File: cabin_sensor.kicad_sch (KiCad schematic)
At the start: 6 parts, among them J5 Внутр. коннектор вентилятора 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, Q2 AO3400

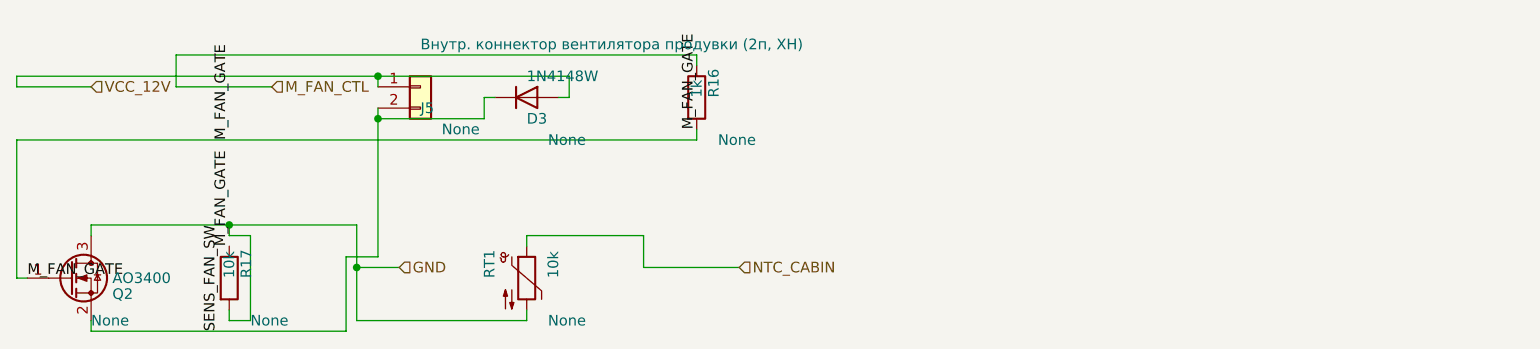
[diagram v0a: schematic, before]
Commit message: all unit test pass
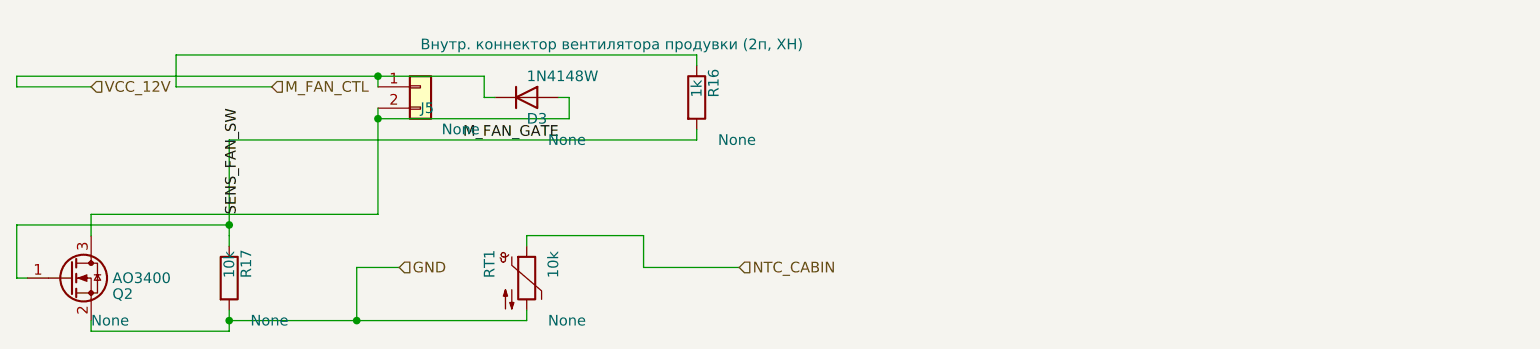
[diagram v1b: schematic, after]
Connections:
- net GND: now also Q2.2 (S); no longer Q2.3 (D)
- net SENS_FAN_SW: now also D3.2 (A), Q2.3 (D); no longer D3.1 (K), Q2.2 (S)
- net VCC_12V: now also D3.1 (K); no longer D3.2 (A)

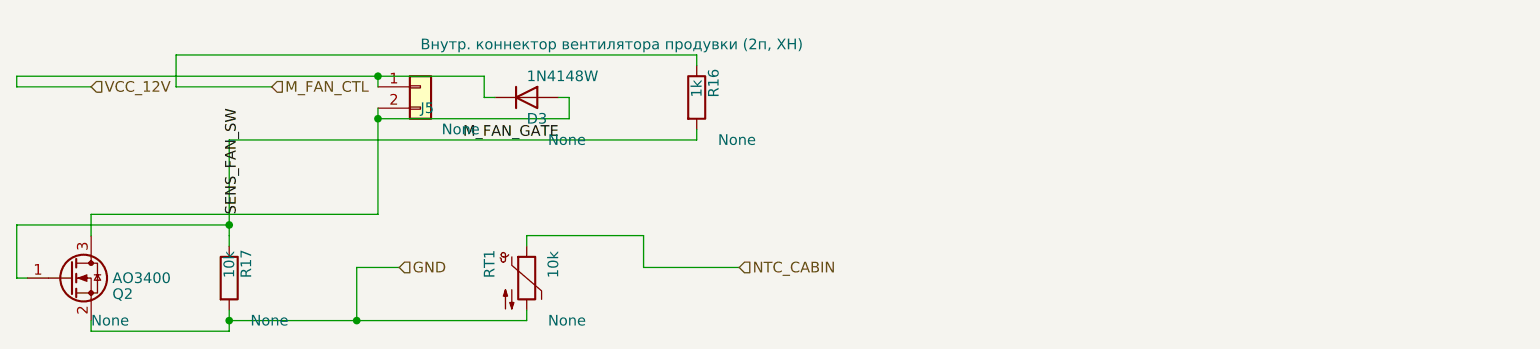
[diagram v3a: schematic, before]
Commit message: tests_fix
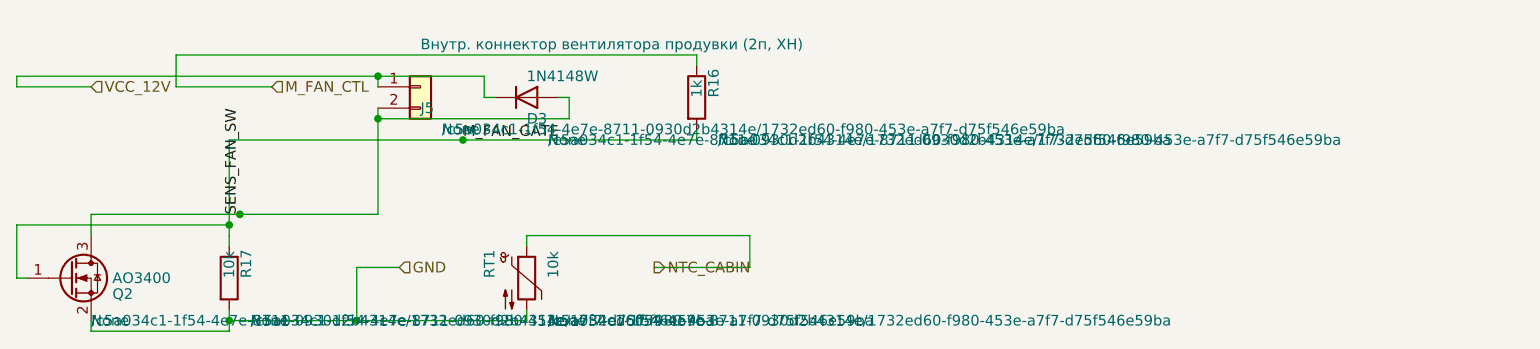
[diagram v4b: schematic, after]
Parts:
- D3, J5, Q2, R16, R17, RT1: hierarchy_path (none) -> /c5a034c1-1f54-4e7e-8711-0930d2b4314e/1732ed60-f980-453e-a7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
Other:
- title: (none) -> climate_control_niva_travel
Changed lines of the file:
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@@
 	(generator_version "9.0")
 	(paper "A4")
+	(title_block
+		(title "climate_control_niva_travel")
+	)
 	(symbol
 		(lib_id "Device:D")
@@
 			)
 		)
+		(property "hierarchy_path" "/c5a034c1-1f54-4e7e-8711-0930d2b4314e/1732ed60-f980-453e-a7f7-d75f546e59ba"
+			(at 66.04 12.6999 0)
+			(effects
+				(font
+					(size 1.27 1.27)
+				)
+				(justify left)
+			)
+		)
 		(pin "1"
 		)
@@
 		)
 		(instances
-			(project "Untitled"
-				(path "/98bb78c5-22b5-4642-853f-3c870b1c4b72"
+			(project "climate_control_niva_travel"
+				(path "/c5a034c1-1f54-4e7e-8711-0930d2b4314e/1732ed60-f980-453e-a7f7-d75f546e59ba"
 					(reference "D3")
 					(unit 1)
@@
 			)
 		)
+		(property "hierarchy_path" "/c5a034c1-1f54-4e7e-8711-0930d2b4314e/1732ed60-f980-453e-a7f7-d75f546e59ba"
+			(at 53.34 11.4299 0)
+			(effects
+				(font
+					(size 1.27 1.27)
+				)
+				(justify left)
+			)
+		)
 		(pin "1"
 		)
@@
 		)
 		(instances
-			(project "Untitled"
-				(path "/98bb78c5-22b5-4642-853f-3c870b1c4b72"
+			(project "climate_control_niva_travel"
+				(path "/c5a034c1-1f54-4e7e-8711-0930d2b4314e/1732ed60-f980-453e-a7f7-d75f546e59ba"
 					(reference "J5")
 					(unit 1)
@@
 			)
 		)
+		(property "hierarchy_path" "/c5a034c1-1f54-4e7e-8711-0930d2b4314e/1732ed60-f980-453e-a7f7-d75f546e59ba"
+			(at 11.43 34.2899 0)
+			(effects
+				(font
+					(size 1.27 1.27)
+				)
+				(justify left)
+			)
+		)
 		(pin "1"
 		)
@@
 		)
 		(instances
-			(project "Untitled"
-				(path "/98bb78c5-22b5-4642-853f-3c870b1c4b72"
+			(project "climate_control_niva_travel"
+				(path "/c5a034c1-1f54-4e7e-8711-0930d2b4314e/1732ed60-f980-453e-a7f7-d75f546e59ba"
 					(reference "Q2")
 					(unit 1)
@@
 			)
 		)
+		(property "hierarchy_path" "/c5a034c1-1f54-4e7e-8711-0930d2b4314e/1732ed60-f980-453e-a7f7-d75f546e59ba"
+			(at 86.36 12.6999 0)
+			(effects
+				(font
+					(size 1.27 1.27)
+				)
+				(justify left)
+			)
+		)
 		(pin "1"
 		)
@@
 		)
 		(instances
-			(project "Untitled"
-				(path "/98bb78c5-22b5-4642-853f-3c870b1c4b72"
+			(project "climate_control_niva_travel"
+				(path "/c5a034c1-1f54-4e7e-8711-0930d2b4314e/1732ed60-f980-453e-a7f7-d75f546e59ba"
 					(reference "R16")
 					(unit 1)
@@
 			)
 		)
+		(property "hierarchy_path" "/c5a034c1-1f54-4e7e-8711-0930d2b4314e/1732ed60-f980-453e-a7f7-d75f546e59ba"
+			(at 30.48 34.2899 0)
+			(effects
+				(font
+					(size 1.27 1.27)
+				)
+				(justify left)
+			)
+		)
 		(pin "1"
 		)
@@
 		)
 		(instances
-			(project "Untitled"
-				(path "/98bb78c5-22b5-4642-853f-3c870b1c4b72"
+			(project "climate_control_niva_travel"
+				(path "/c5a034c1-1f54-4e7e-8711-0930d2b4314e/1732ed60-f980-453e-a7f7-d75f546e59ba"
 					(reference "R17")
 					(unit 1)
@@
 			)
 		)
+		(property "hierarchy_path" "/c5a034c1-1f54-4e7e-8711-0930d2b4314e/1732ed60-f980-453e-a7f7-d75f546e59ba"
+			(at 66.04 34.2899 0)
+			(effects
+				(font
+					(size 1.27 1.27)
+				)
+				(justify left)
+			)
+		)
 		(pin "1"
 		)
@@
 		)
 		(instances
-			(project "Untitled"
-				(path "/98bb78c5-22b5-4642-853f-3c870b1c4b72"
+			(project "climate_control_niva_travel"
+				(path "/c5a034c1-1f54-4e7e-8711-0930d2b4314e/1732ed60-f980-453e-a7f7-d75f546e59ba"
 					(reference "RT1")
 					(unit 1)
@@
 	(wire
 		(pts
-			(xy 63.5 24.13) (xy 77.47 24.13)
-		)
-		(stroke
-			(width 0)
-			(type default)
-		)
-	)
-	(wire
-		(pts
-			(xy 77.47 24.13) (xy 77.47 27.94)
-		)
-		(stroke
-			(width 0)
-			(type default)
-		)
-	)
-	(wire
-		(pts
-			(xy 77.47 27.94) (xy 88.9 27.94)
+			(xy 63.5 24.13) (xy 90.17 24.13)
+		)
+		(stroke
+			(width 0)
+			(type default)
+		)
+	)
+	(wire
+		(pts
+			(xy 90.17 24.13) (xy 90.17 27.94)
+		)
+		(stroke
+			(width 0)
+			(type default)
+		)
+	)
+	(wire
+		(pts
+			(xy 90.17 27.94) (xy 78.74 27.94)
 		)
 		(stroke
@@
 	(junction
 		(at 45.72 10.16)
+		(diameter 0)
+		(color 0 0 0 0)
+	)
+	(junction
+		(at 55.88 12.7)
+		(diameter 0)
+		(color 0 0 0 0)
+	)
+	(junction
+		(at 29.21 21.59)
 		(diameter 0)
 		(color 0 0 0 0)
@@
 	)
 	(hierarchical_label "NTC_CABIN"
-		(shape input)
-		(at 88.9 27.94 180)
+		(shape output)
+		(at 78.74 27.94 0)
 		(effects
 			(font

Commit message: refactoring
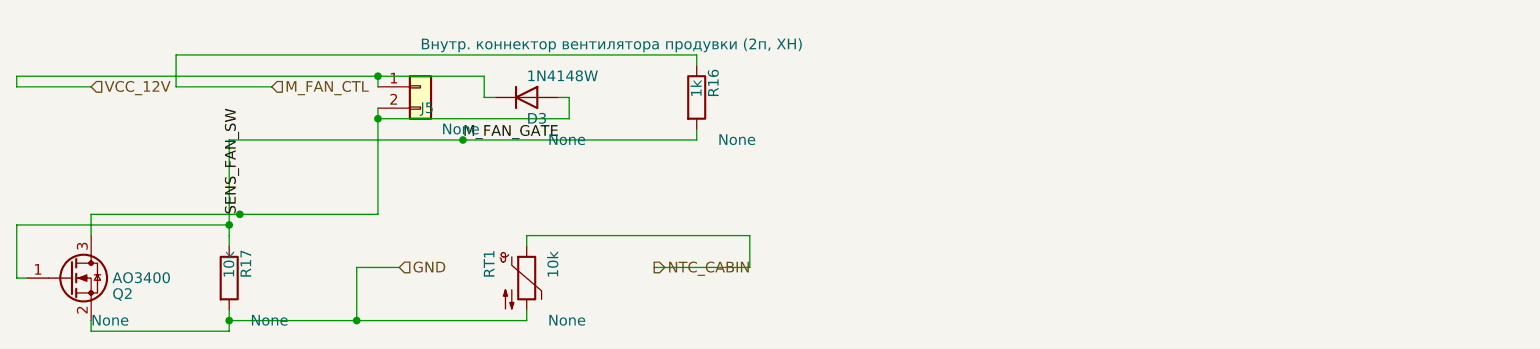
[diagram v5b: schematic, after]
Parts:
- D3, J5, Q2, R16, R17, RT1: hierarchy_path /c5a034c1-1f54-4e7e-8711-0930d2b4314e/1732ed60-f980-453e-a7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 -> (none)
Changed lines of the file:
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@@
 			)
 		)
-		(property "hierarchy_path" "/c5a034c1-1f54-4e7e-8711-0930d2b4314e/1732ed60-f980-453e-a7f7-d75f546e59ba"
-			(at 66.04 12.6999 0)
-			(effects
-				(font
-					(size 1.27 1.27)
-				)
-				(justify left)
-			)
-		)
-		(pin "1"
-		)
-		(pin "2"
-		)
-		(instances
-			(project "climate_control_niva_travel"
-				(path "/c5a034c1-1f54-4e7e-8711-0930d2b4314e/1732ed60-f980-453e-a7f7-d75f546e59ba"
-					(reference "D3")
+		(pin "1"
+		)
+		(pin "2"
+		)
+		(instances
+			(project "climate_control_niva_travel"
+				(path "/165a98f1-2dde-4141-9fdc-c935d39c8cff/1511d7be-6bc1-43c4-af0e-a2c3e148ee38/"
+					(reference "D0903")
 					(unit 1)
 				)
@@
 			)
 		)
-		(property "hierarchy_path" "/c5a034c1-1f54-4e7e-8711-0930d2b4314e/1732ed60-f980-453e-a7f7-d75f546e59ba"
-			(at 53.34 11.4299 0)
-			(effects
-				(font
-					(size 1.27 1.27)
-				)
-				(justify left)
-			)
-		)
-		(pin "1"
-		)
-		(pin "2"
-		)
-		(instances
-			(project "climate_control_niva_travel"
-				(path "/c5a034c1-1f54-4e7e-8711-0930d2b4314e/1732ed60-f980-453e-a7f7-d75f546e59ba"
-					(reference "J5")
+		(pin "1"
+		)
+		(pin "2"
+		)
+		(instances
+			(project "climate_control_niva_travel"
+				(path "/165a98f1-2dde-4141-9fdc-c935d39c8cff/1511d7be-6bc1-43c4-af0e-a2c3e148ee38/"
+					(reference "J0905")
 					(unit 1)
 				)
@@
 			)
 		)
-		(property "hierarchy_path" "/c5a034c1-1f54-4e7e-8711-0930d2b4314e/1732ed60-f980-453e-a7f7-d75f546e59ba"
-			(at 11.43 34.2899 0)
-			(effects
-				(font
-					(size 1.27 1.27)
-				)
-				(justify left)
-			)
-		)
 		(pin "1"
 		)
@@
 		(instances
 			(project "climate_control_niva_travel"
-				(path "/c5a034c1-1f54-4e7e-8711-0930d2b4314e/1732ed60-f980-453e-a7f7-d75f546e59ba"
-					(reference "Q2")
+				(path "/165a98f1-2dde-4141-9fdc-c935d39c8cff/1511d7be-6bc1-43c4-af0e-a2c3e148ee38/"
+					(reference "Q0902")
 					(unit 1)
 				)
@@
 			)
 		)
-		(property "hierarchy_path" "/c5a034c1-1f54-4e7e-8711-0930d2b4314e/1732ed60-f980-453e-a7f7-d75f546e59ba"
-			(at 86.36 12.6999 0)
-			(effects
-				(font
-					(size 1.27 1.27)
-				)
-				(justify left)
-			)
-		)
-		(pin "1"
-		)
-		(pin "2"
-		)
-		(instances
-			(project "climate_control_niva_travel"
-				(path "/c5a034c1-1f54-4e7e-8711-0930d2b4314e/1732ed60-f980-453e-a7f7-d75f546e59ba"
-					(reference "R16")
+		(pin "1"
+		)
+		(pin "2"
+		)
+		(instances
+			(project "climate_control_niva_travel"
+				(path "/165a98f1-2dde-4141-9fdc-c935d39c8cff/1511d7be-6bc1-43c4-af0e-a2c3e148ee38/"
+					(reference "R0916")
 					(unit 1)
 				)
@@
 			)
 		)
-		(property "hierarchy_path" "/c5a034c1-1f54-4e7e-8711-0930d2b4314e/1732ed60-f980-453e-a7f7-d75f546e59ba"
-			(at 30.48 34.2899 0)
-			(effects
-				(font
-					(size 1.27 1.27)
-				)
-				(justify left)
-			)
-		)
-		(pin "1"
-		)
-		(pin "2"
-		)
-		(instances
-			(project "climate_control_niva_travel"
-				(path "/c5a034c1-1f54-4e7e-8711-0930d2b4314e/1732ed60-f980-453e-a7f7-d75f546e59ba"
-					(reference "R17")
+		(pin "1"
+		)
+		(pin "2"
+		)
+		(instances
+			(project "climate_control_niva_travel"
+				(path "/165a98f1-2dde-4141-9fdc-c935d39c8cff/1511d7be-6bc1-43c4-af0e-a2c3e148ee38/"
+					(reference "R0917")
 					(unit 1)
 				)
@@
 			)
 		)
-		(property "hierarchy_path" "/c5a034c1-1f54-4e7e-8711-0930d2b4314e/1732ed60-f980-453e-a7f7-d75f546e59ba"
-			(at 66.04 34.2899 0)
-			(effects
-				(font
-					(size 1.27 1.27)
-				)
-				(justify left)
-			)
-		)
-		(pin "1"
-		)
-		(pin "2"
-		)
-		(instances
-			(project "climate_control_niva_travel"
-				(path "/c5a034c1-1f54-4e7e-8711-0930d2b4314e/1732ed60-f980-453e-a7f7-d75f546e59ba"
-					(reference "RT1")
-					(unit 1)
-				)
+		(pin "1"
+		)
+		(pin "2"
+		)
+		(instances
+			(project "climate_control_niva_travel"
+				(path "/165a98f1-2dde-4141-9fdc-c935d39c8cff/1511d7be-6bc1-43c4-af0e-a2c3e148ee38/"
+					(reference "RT0901")
+					(unit 1)
+				)

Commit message: refactoring
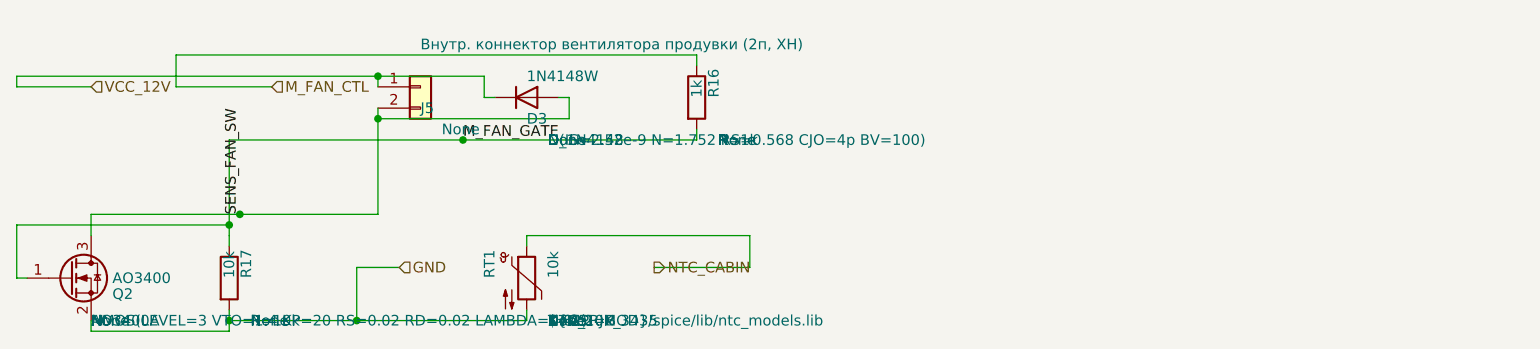
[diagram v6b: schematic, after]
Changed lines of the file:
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@@
+			)
+		)
+		(property "Sim.Device" "D"
+			(at 66.04 12.6999 0)
+			(effects
+				(font
+					(size 1.27 1.27)
+				)
+				(justify left)
+			)
+		)
+		(property "Sim.Model" "D_1N4148"
+			(at 66.04 12.6999 0)
+			(effects
+				(font
+					(size 1.27 1.27)
+				)
+				(justify left)
+			)
+		)
+		(property "Sim.Params" "D(IS=2.52e-9 N=1.752 RS=0.568 CJO=4p BV=100)"
+			(at 66.04 12.6999 0)
+			(effects
+				(font
+					(size 1.27 1.27)
+				)
+				(justify left)
 			)
 		)
@@
 		(instances
 			(project "climate_control_niva_travel"
-				(path "/165a98f1-2dde-4141-9fdc-c935d39c8cff/1511d7be-6bc1-43c4-af0e-a2c3e148ee38/"
+				(path "/cc416b40-1361-4232-ac1e-5cd36ef0c0fb/5e27c952-8344-432b-b815-f24e34f2b050/"
 					(reference "D0903")
 					(unit 1)
@@
 		(instances
 			(project "climate_control_niva_travel"
-				(path "/165a98f1-2dde-4141-9fdc-c935d39c8cff/1511d7be-6bc1-43c4-af0e-a2c3e148ee38/"
+				(path "/cc416b40-1361-4232-ac1e-5cd36ef0c0fb/5e27c952-8344-432b-b815-f24e34f2b050/"
 					(reference "J0905")
 					(unit 1)
@@
 			)
 		)
+		(property "Sim.Device" "M"
+			(at 11.43 34.2899 0)
+			(effects
+				(font
+					(size 1.27 1.27)
+				)
+				(justify left)
+			)
+		)
+		(property "Sim.Model" "AO3400A"
+			(at 11.43 34.2899 0)
+			(effects
+				(font
+					(size 1.27 1.27)
+				)
+				(justify left)
+			)
+		)
+		(property "Sim.Params" "NMOS(LEVEL=3 VTO=1.4 KP=20 RS=0.02 RD=0.02 LAMBDA=0.02)"
+			(at 11.43 34.2899 0)
+			(effects
+				(font
+					(size 1.27 1.27)
+				)
+				(justify left)
+			)
+		)
 		(pin "1"
 		)
@@
 		(instances
 			(project "climate_control_niva_travel"
-				(path "/165a98f1-2dde-4141-9fdc-c935d39c8cff/1511d7be-6bc1-43c4-af0e-a2c3e148ee38/"
+				(path "/cc416b40-1361-4232-ac1e-5cd36ef0c0fb/5e27c952-8344-432b-b815-f24e34f2b050/"
 					(reference "Q0902")
 					(unit 1)
@@
 			)
 		)
+		(property "Sim.Device" "R"
+			(at 86.36 12.6999 0)
+			(effects
+				(font
+					(size 1.27 1.27)
+				)
+				(justify left)
+			)
+		)
+		(property "Sim.Params" "R=1k"
+			(at 86.36 12.6999 0)
+			(effects
+				(font
+					(size 1.27 1.27)
+				)
+				(justify left)
+			)
+		)
 		(pin "1"
 		)
@@
 		(instances
 			(project "climate_control_niva_travel"
-				(path "/165a98f1-2dde-4141-9fdc-c935d39c8cff/1511d7be-6bc1-43c4-af0e-a2c3e148ee38/"
+				(path "/cc416b40-1361-4232-ac1e-5cd36ef0c0fb/5e27c952-8344-432b-b815-f24e34f2b050/"
 					(reference "R0916")
 					(unit 1)
@@
 			)
 		)
+		(property "Sim.Device" "R"
+			(at 30.48 34.2899 0)
+			(effects
+				(font
+					(size 1.27 1.27)
+				)
+				(justify left)
+			)
+		)
+		(property "Sim.Params" "R=10k"
+			(at 30.48 34.2899 0)
+			(effects
+				(font
+					(size 1.27 1.27)
+				)
+				(justify left)
+			)
+		)
 		(pin "1"
 		)
@@
 		(instances
 			(project "climate_control_niva_travel"
-				(path "/165a98f1-2dde-4141-9fdc-c935d39c8cff/1511d7be-6bc1-43c4-af0e-a2c3e148ee38/"
+				(path "/cc416b40-1361-4232-ac1e-5cd36ef0c0fb/5e27c952-8344-432b-b815-f24e34f2b050/"
 					(reference "R0917")
 					(unit 1)
@@
 			)
 		)
+		(property "Sim.Device" "X"
+			(at 66.04 34.2899 0)
+			(effects
+				(font
+					(size 1.27 1.27)
+				)
+				(justify left)
+			)
+		)
+		(property "Sim.Name" "NTC_10K_3435"
+			(at 66.04 34.2899 0)
+			(effects
+				(font
+					(size 1.27 1.27)
+				)
+				(justify left)
+			)
+		)
+		(property "Sim.Library" "${KIPRJMOD}/spice/lib/ntc_models.lib"
+			(at 66.04 34.2899 0)
+			(effects
+				(font
+					(size 1.27 1.27)
+				)
+				(justify left)
+			)
+		)
+		(property "Sim.Pins" "1=A 2=B"
+			(at 66.04 34.2899 0)
+			(effects
+				(font
+					(size 1.27 1.27)
+				)
+				(justify left)
+			)
+		)
+		(property "Sim.Params" "T=25"
+			(at 66.04 34.2899 0)
+			(effects
+				(font
+					(size 1.27 1.27)
+				)
+				(justify left)
+			)
+		)
+		(property "Sim.Enable" "1"
+			(at 66.04 34.2899 0)
+			(effects
+				(font
+					(size 1.27 1.27)
+				)
+				(justify left)
+			)
+		)
 		(pin "1"
 		)
@@
 		(instances
 			(project "climate_control_niva_travel"
-				(path "/165a98f1-2dde-4141-9fdc-c935d39c8cff/1511d7be-6bc1-43c4-af0e-a2c3e148ee38/"
+				(path "/cc416b40-1361-4232-ac1e-5cd36ef0c0fb/5e27c952-8344-432b-b815-f24e34f2b050/"
 					(reference "RT0901")
 					(unit 1)
@@
 	(junction
 		(at 45.72 5.08)
-		(diameter 0)
+		(diameter 0.0000)
 		(color 0 0 0 0)
 	)
 	(junction
 		(at 27.94 34.29)
-		(diameter 0)
+		(diameter 0.0000)
 		(color 0 0 0 0)
 	)
 	(junction
 		(at 43.18 34.29)
-		(diameter 0)
+		(diameter 0.0000)
 		(color 0 0 0 0)
 	)
 	(junction
 		(at 27.94 22.86)
-		(diameter 0)
+		(diameter 0.0000)
 		(color 0 0 0 0)
 	)
 	(junction
 		(at 45.72 10.16)
-		(diameter 0)
+		(diameter 0.0000)
 		(color 0 0 0 0)
 	)
 	(junction
 		(at 55.88 12.7)
-		(diameter 0)
+		(diameter 0.0000)
 		(color 0 0 0 0)
 	)
 	(junction
 		(at 29.21 21.59)
-		(diameter 0)
+		(diameter 0.0000)
 		(color 0 0 0 0)
 	)
